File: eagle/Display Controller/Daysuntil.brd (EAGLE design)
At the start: 45 parts, among them IC1 DS1307, IC2 ATMEGA168-20P, IC3 74HC595N, IC4 74HC595N, IC5 7805TV, Q1 32.768 kHz, T1 BC337, T10 BC337, T11 BC337, T12 BC337, T13 BC337, T14 BC337, T2 BC337, T3 BC337, T4 BC337, T5 BC337, T6 BC337, T7 BC337, T8 BC337, T9 BC337

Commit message: updated board config
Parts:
- C1, C4, C5, C6: value 10uF -> 0.1uF
- C2, C3: value 10uF -> 100uF
- U$2: value (none) -> 16MHz
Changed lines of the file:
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@@
 <attribute name="VALUE" x="66.9798" y="40.132" size="1.778" layer="27" ratio="10" rot="R90"/>
 </element>
-<element name="U$2" library="adafruit" package="CERM_OSC" value="" x="46.99" y="33.02" smashed="yes" rot="R180">
+<element name="U$2" library="adafruit" package="CERM_OSC" value="16MHz" x="46.99" y="33.02" smashed="yes" rot="R180">
 <attribute name="VALUE" x="50.49" y="37.52" size="1.27" layer="27" rot="R180"/>
 </element>
@@
 <attribute name="VALUE" x="27.94" y="26.67" size="1.27" layer="27" ratio="10" rot="R90"/>
 </element>
-<element name="C2" library="adafruit" package="C050-050X075" value="10uF" x="22.86" y="27.94" smashed="yes" rot="R270">
+<element name="C2" library="adafruit" package="C050-050X075" value="100uF" x="22.86" y="27.94" smashed="yes" rot="R270">
 <attribute name="NAME" x="22.479" y="23.749" size="1.27" layer="25" ratio="10" rot="R180"/>
 <attribute name="VALUE" x="20.701" y="31.115" size="1.27" layer="27" ratio="10" rot="R270"/>
 </element>
-<element name="C3" library="adafruit" package="C050-050X075" value="10uF" x="36.83" y="31.75" smashed="yes" rot="R90">
+<element name="C3" library="adafruit" package="C050-050X075" value="100uF" x="36.83" y="31.75" smashed="yes" rot="R90">
 <attribute name="NAME" x="37.719" y="27.559" size="1.27" layer="25" ratio="10" rot="R180"/>
 <attribute name="VALUE" x="38.989" y="28.575" size="1.27" layer="27" ratio="10" rot="R90"/>
 </element>
 <element name="JP1" library="pinhead" package="1X16" value="Output" x="17.78" y="46.99" rot="R270"/>
-<element name="C1" library="adafruit" package="C025-030X050" value="10uF" x="67.31" y="68.58" smashed="yes">
+<element name="C1" library="adafruit" package="C025-030X050" value="0.1uF" x="67.31" y="68.58" smashed="yes">
 <attribute name="NAME" x="66.294" y="70.485" size="1.27" layer="25" ratio="10"/>
 <attribute name="VALUE" x="65.024" y="65.532" size="1.27" layer="27" ratio="10"/>
 </element>
-<element name="C4" library="adafruit" package="C025-030X050" value="10uF" x="40.64" y="24.13" smashed="yes" rot="R270">
+<element name="C4" library="adafruit" package="C025-030X050" value="0.1uF" x="40.64" y="24.13" smashed="yes" rot="R270">
 <attribute name="NAME" x="39.624" y="27.305" size="1.27" layer="25" ratio="10"/>
 <attribute name="VALUE" x="38.354" y="19.812" size="1.27" layer="27" ratio="10"/>
 </element>
-<element name="C6" library="adafruit" package="C025-030X050" value="10uF" x="35.56" y="52.07" smashed="yes" rot="R90">
+<element name="C6" library="adafruit" package="C025-030X050" value="0.1uF" x="35.56" y="52.07" smashed="yes" rot="R90">
 <attribute name="NAME" x="38.735" y="48.514" size="1.27" layer="25" ratio="10" rot="R90"/>
 <attribute name="VALUE" x="38.608" y="52.324" size="1.27" layer="27" ratio="10" rot="R90"/>
 </element>
-<element name="C5" library="adafruit" package="C025-030X050" value="10uF" x="35.56" y="40.64" smashed="yes" rot="R90">
+<element name="C5" library="adafruit" package="C025-030X050" value="0.1uF" x="35.56" y="40.64" smashed="yes" rot="R90">
 <attribute name="NAME" x="38.735" y="37.084" size="1.27" layer="25" ratio="10" rot="R90"/>
 <attribute name="VALUE" x="38.608" y="40.894" size="1.27" layer="27" ratio="10" rot="R90"/>

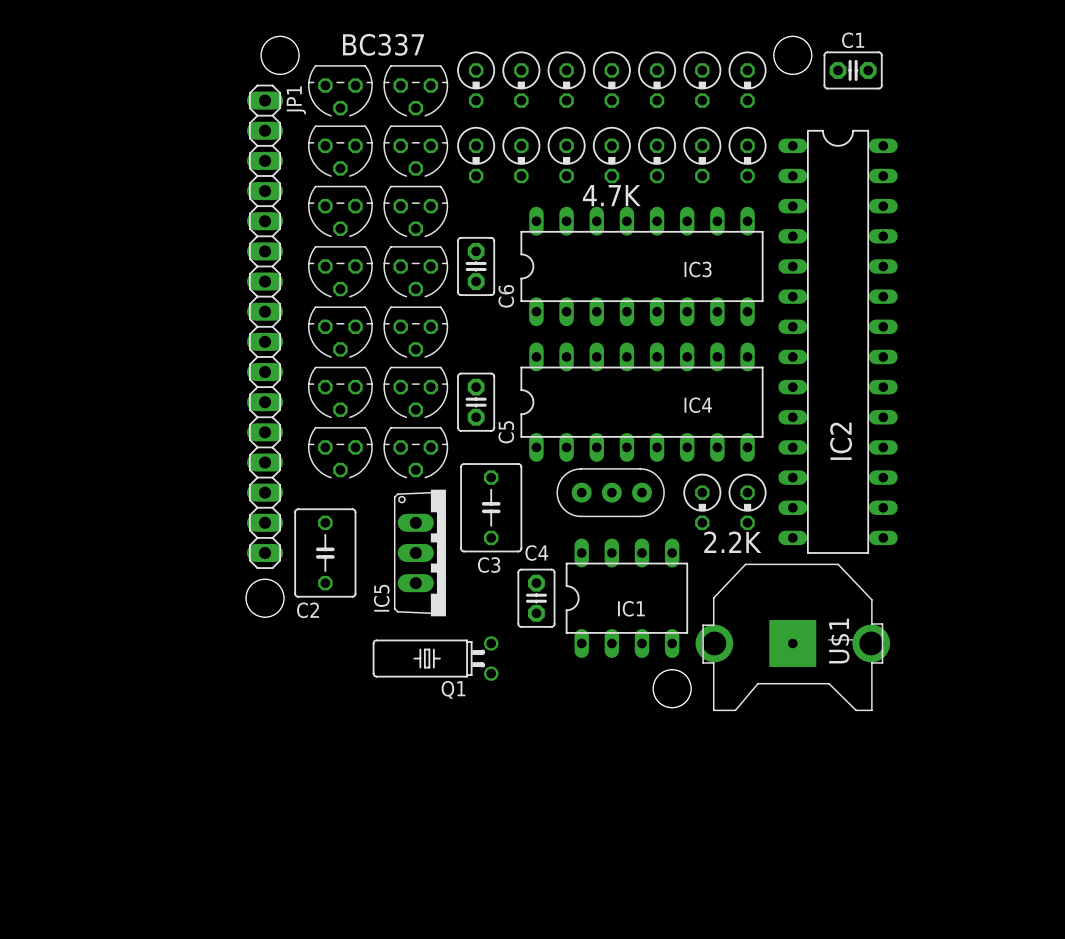
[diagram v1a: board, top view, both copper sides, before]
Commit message: finalized board design
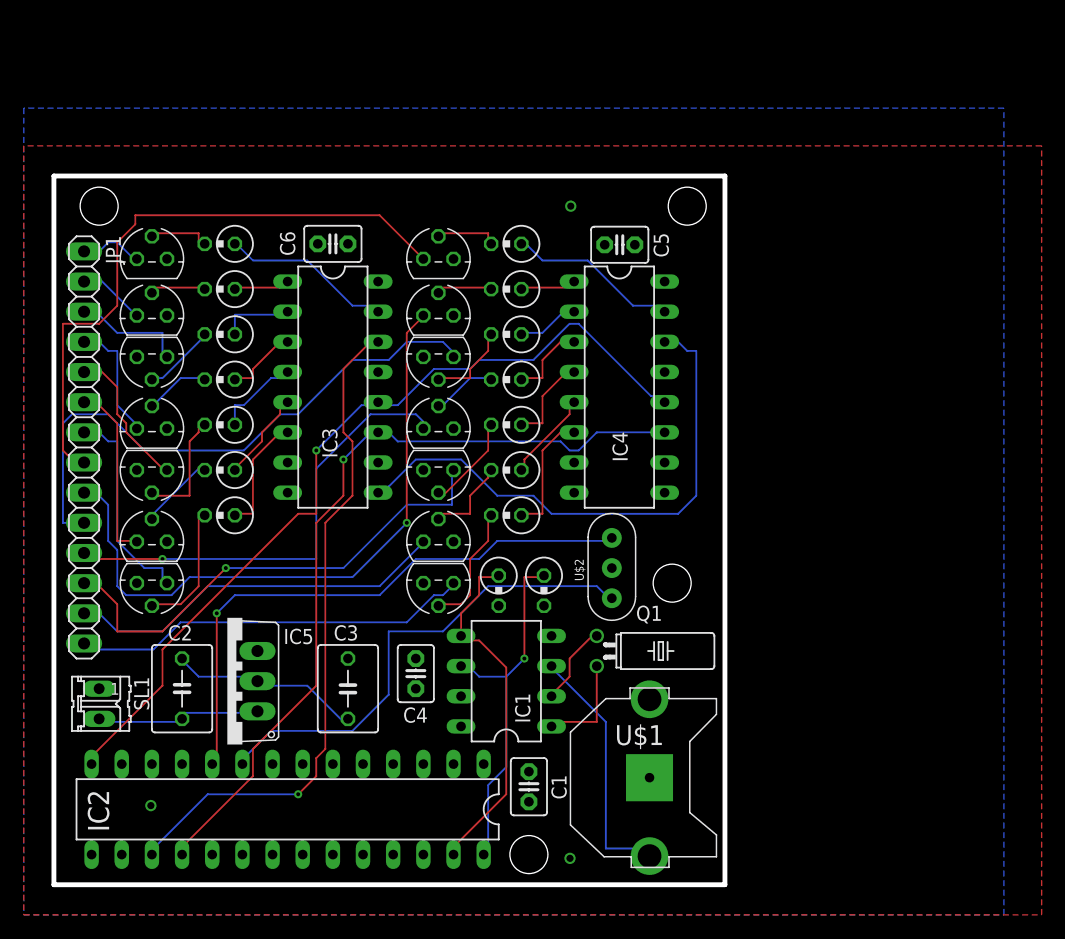
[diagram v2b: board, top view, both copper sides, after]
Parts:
- added SL1: (no value), con-amp-quick:02P
- IC2: value ATMEGA168-20P -> ATMEGA328P
- JP1: value Output -> (none); device pinhead:1X16 -> pinhead:1X14
- moved C1 66.2 mm to (40.0, 8.26), turned to 270 degrees
- moved IC2 60.8 mm to (19.7, 6.35), turned to 180 degrees
- moved R9 57.3 mm to (14.0, 31.1), turned to 180 degrees
- moved R8 52.0 mm to (14.0, 34.9), turned to 180 degrees
- moved R7 46.6 mm to (14.0, 38.7), turned to 180 degrees
- moved R6 41.3 mm to (14.0, 42.5), turned to 180 degrees
- moved R16 36.1 mm to (38.1, 31.1), turned to 180 degrees
- moved T6 36.0 mm to (8.26, 28.9), turned to 0 degrees
- moved R5 35.9 mm to (14.0, 46.4), turned to 180 degrees
- moved T4 32.6 mm to (8.26, 38.4), turned to 0 degrees
- moved T7 31.0 mm to (8.26, 25.4)
- moved R15 30.8 mm to (38.1, 34.9), turned to 180 degrees
- moved R4 30.6 mm to (14.0, 50.2), turned to 180 degrees
- moved T2 29.5 mm to (8.26, 47.9), turned to 0 degrees
- moved IC3 27.9 mm to (23.5, 41.9), turned to 270 degrees
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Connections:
- net +12V: now also SL1.2; no longer JP1.16
- net GND: now also SL1.1; no longer JP1.15
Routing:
- net N$7: track 0.00 -> 72.0 mm, vias 0 -> 1
- net N$6: track 0.00 -> 68.2 mm, vias 0 -> 1
- net N$2: track 0.00 -> 56.5 mm, vias 0 -> 1
- net 9: track 0.00 -> 55.1 mm, vias 0 -> 1
- net 8: track 0.00 -> 52.8 mm
- net 10: track 0.00 -> 49.1 mm
- net N$9: track 0.00 -> 48.7 mm, vias 0 -> 1
- net SER: track 0.00 -> 45.8 mm
- net 12: track 0.00 -> 42.1 mm, vias 0 -> 1
- net N$8: track 0.00 -> 41.0 mm
- net 11: track 0.00 -> 39.2 mm, vias 0 -> 1
- net 14: track 0.00 -> 33.7 mm
- net 13: track 0.00 -> 32.6 mm
- net SCL: track 0.00 -> 30.7 mm, vias 0 -> 1
- net SDA: track 0.00 -> 30.1 mm
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- added copper zone on layer 1, net GND
- added copper zone on layer 16, net VCC
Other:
- board outline added: 56.5 x 59.7 mm
- board text added: "/home/brian/Pictures/Images/santa1.bmp"
- board text added: "1"
- board text added: "RTC Display v1.0"
- board text added: "wilsonb@outlook.com"
- board text removed: "2.2K"
- board text removed: "4.7K"
- board text removed: "BC337"
